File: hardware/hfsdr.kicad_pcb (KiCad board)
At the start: 2 copper layers, 100 x 99.4 mm, 82 parts, among them J1 USB_C_Receptacle_USB2.0_16P, Q1 AO3401A, SW1 RST, SW2 BOOT0, U1 SN74CBT3253, U2 XLV320ADC6120IRTER, U3 CH32V30xRxTx, U4 MD57E33QA3, U5 MD57E33QA3, U6 BGA2817, U7 TP4054, U8 LM4809, X1 2T024000VX, Y1 Si5351A-B-GT

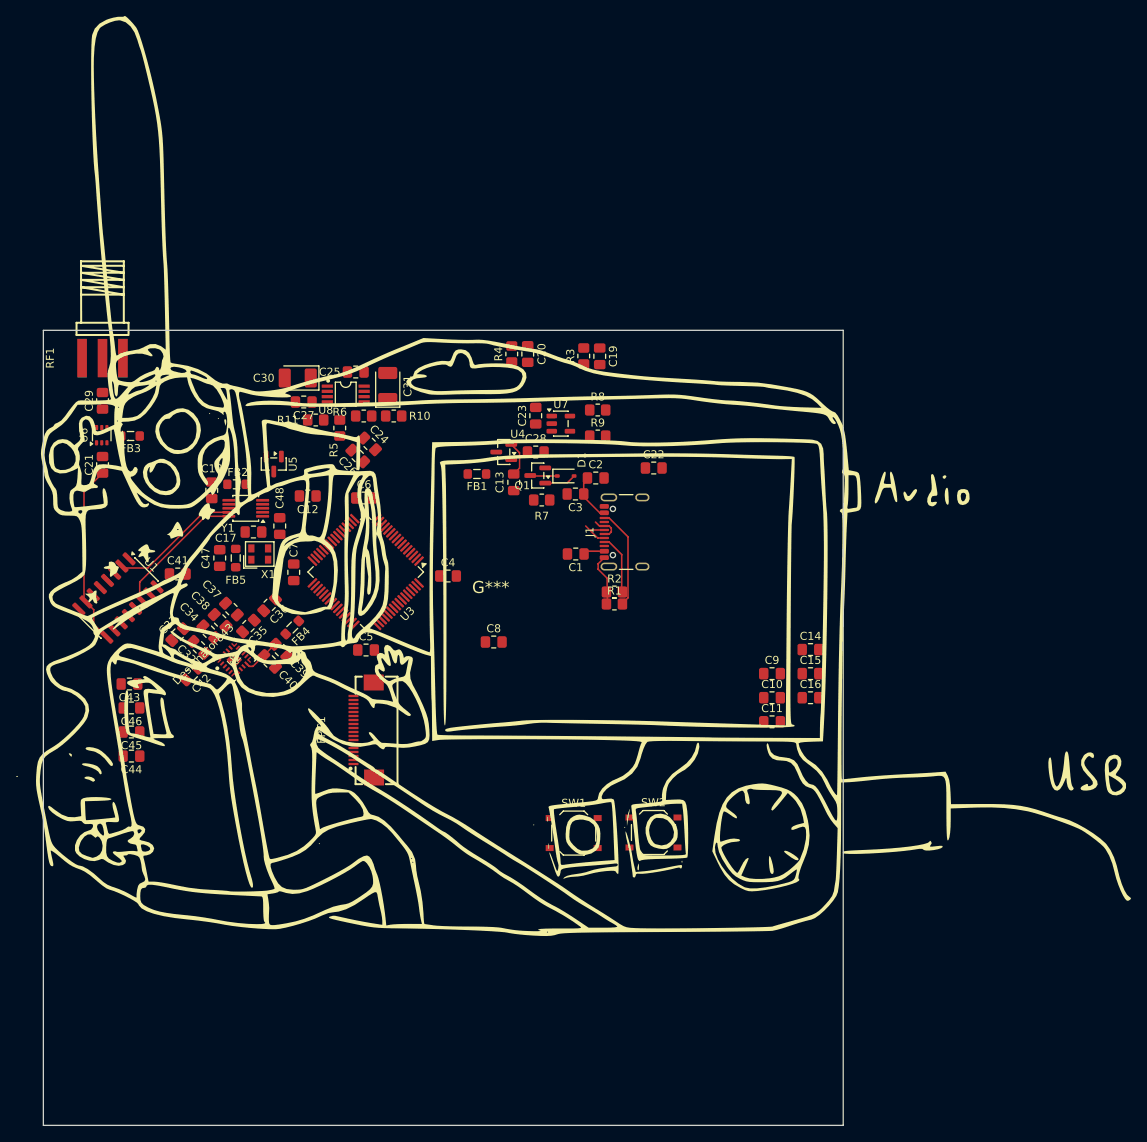
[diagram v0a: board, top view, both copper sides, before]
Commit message: layout + some routing
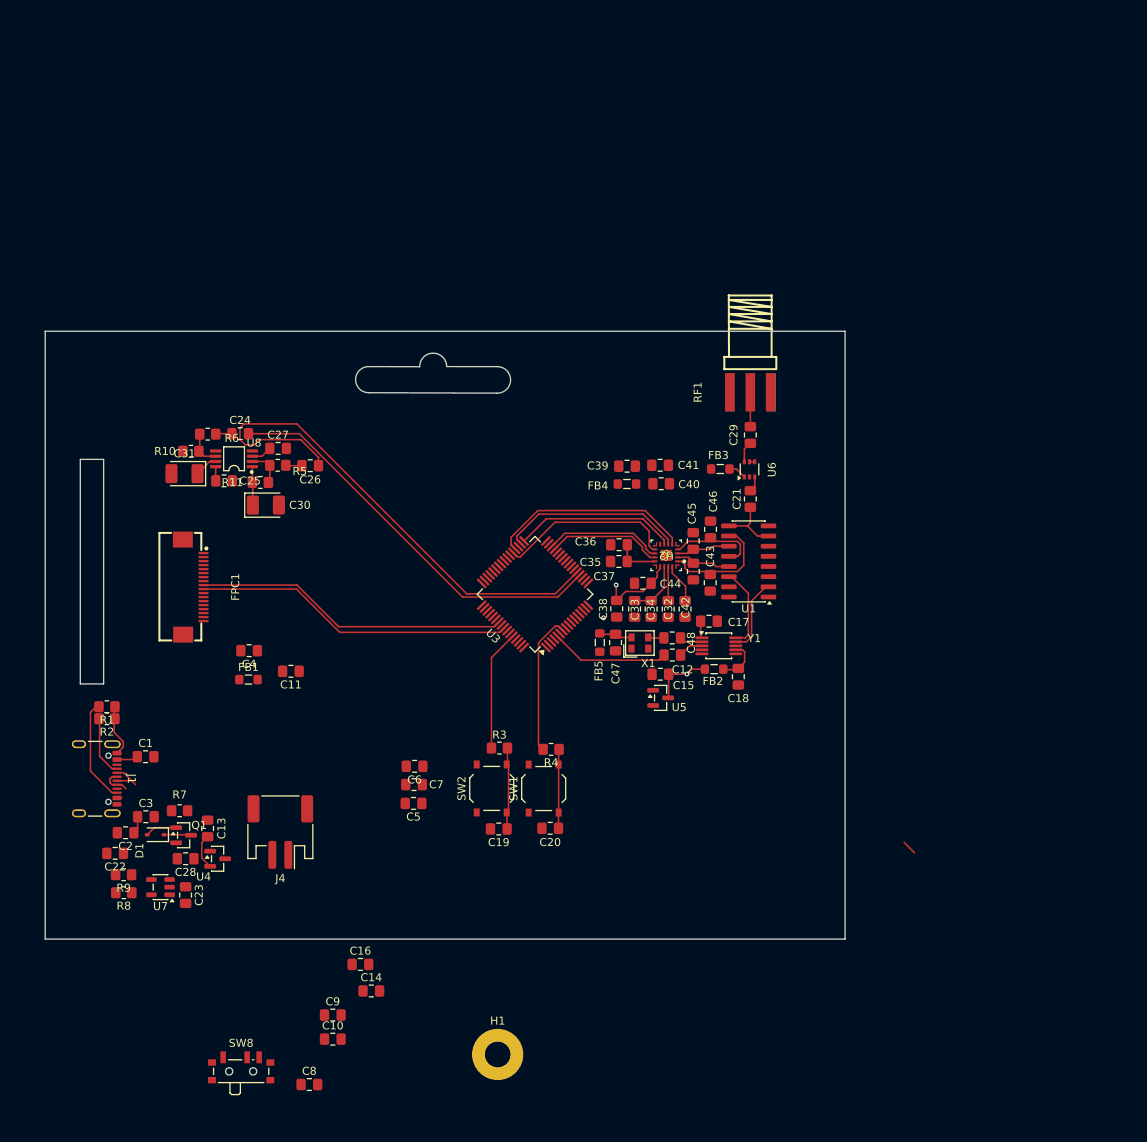
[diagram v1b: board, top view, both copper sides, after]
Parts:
- added H1: MountingHole_Pad, MountingHole:MountingHole_3.2mm_M3_Pad, F.Cu at (118.5, 125.8)
- added J4: JST PH S2B, Connector_JST:JST_PH_S2B-PH-SM4-TB_1x02-1MP_P2.00mm_Horizontal, F.Cu at (91.3, 98.0)
- added SW8: SW_SPDT, Button_Switch_SMD:SW_SPDT_PCM12, F.Cu at (86.4, 127.6)
- G***: moved to B.Cu
- moved R8 84.6 mm to (71.8, 105.6), turned to 180 degrees
- moved C22 82.8 mm to (70.7, 100.7), turned to 180 degrees
- moved C21 81.1 mm to (150.1, 56.4)
- moved C29 81.1 mm to (150.1, 48.4)
- moved RF1 81.1 mm to (150.1, 43.0)
- moved U6 81.1 mm to (150.0, 52.7)
- moved R9 80.7 mm to (71.7, 103.3), turned to 180 degrees
- moved U1 79.0 mm to (149.9, 64.2), turned to 180 degrees
- moved U7 76.6 mm to (76.3, 104.9), turned to 180 degrees
- moved C46 75.7 mm to (145.1, 60.2), turned to -90 degrees
- moved J1 74.9 mm to (67.2, 91.3), turned to -90 degrees
- moved C23 74.2 mm to (79.5, 105.9), turned to -90 degrees
- moved C45 74.2 mm to (142.9, 61.6), turned to -90 degrees
- moved C44 73.9 mm to (143.0, 65.4), turned to 90 degrees
- moved FB3 73.8 mm to (146.3, 52.6), turned to 0 degrees
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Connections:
- C20 pad 2: Net-(SW1-A) -> Net-(SW1-B)
- C28 pad 1: +5V -> Net-(D1-K)
- D1 pad 1: +5V -> Net-(D1-K)
- Q1 pad 3: +5V -> Net-(D1-K)
- R4 pad 1: +3.3V -> Net-(SW1-B)
- SW1 pad 1: Net-(SW1-A) -> +3.3V
- SW1 pad 2: +3.3V -> Net-(SW1-B)
- U3 pad 46: unconnected-(U3-SWDIO-Pad46) -> SWDIO
- U3 pad 49: unconnected-(U3-SWCLK-Pad49) -> SWCLK
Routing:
- net DAC2_OUT: track 0.00 -> 66.0 mm
- net DAC1_OUT: track 0.00 -> 51.0 mm
- net SDA_MOSI: track 0.00 -> 40.1 mm
- net SCL_SCK: track 0.00 -> 39.3 mm
- net SD: track 0.00 -> 25.5 mm
- net CK: track 0.00 -> 23.2 mm
- net MCK: track 0.00 -> 22.3 mm
- net WS: track 0.00 -> 20.3 mm
- net Net-(U3-~{RST}): track 0.00 -> 17.7 mm
- net +3.3VA: track 0.00 -> 17.5 mm, vias 0 -> 2
- net Net-(U3-OSC_IN): track 0.00 -> 17.2 mm
- net Net-(U3-BOOT0): track 0.00 -> 15.1 mm
- net SDA: track 0.00 -> 14.9 mm
- net SCL: track 0.00 -> 14.5 mm
- net Net-(U1-2B1): track 0.00 -> 14.4 mm
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- added copper zone on In2.Cu, net +3.3V
- added copper zone on In2.Cu, net +3.3VA
- added copper zone on In1.Cu, net GND
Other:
- board size 100 x 99.4 mm -> 100 x 76 mm
- copper layers 2 -> 4
